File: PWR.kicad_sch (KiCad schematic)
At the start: 22 parts, among them J1 Conn_01x04_Pin, J2 Conn_01x03_Pin, J3 Conn_01x03_Pin, J4 Conn_01x03_Pin, J5 Conn_01x03_Pin, J6 Conn_01x04_Pin, U1 LM66100DCK, U2 XC6206P332MR

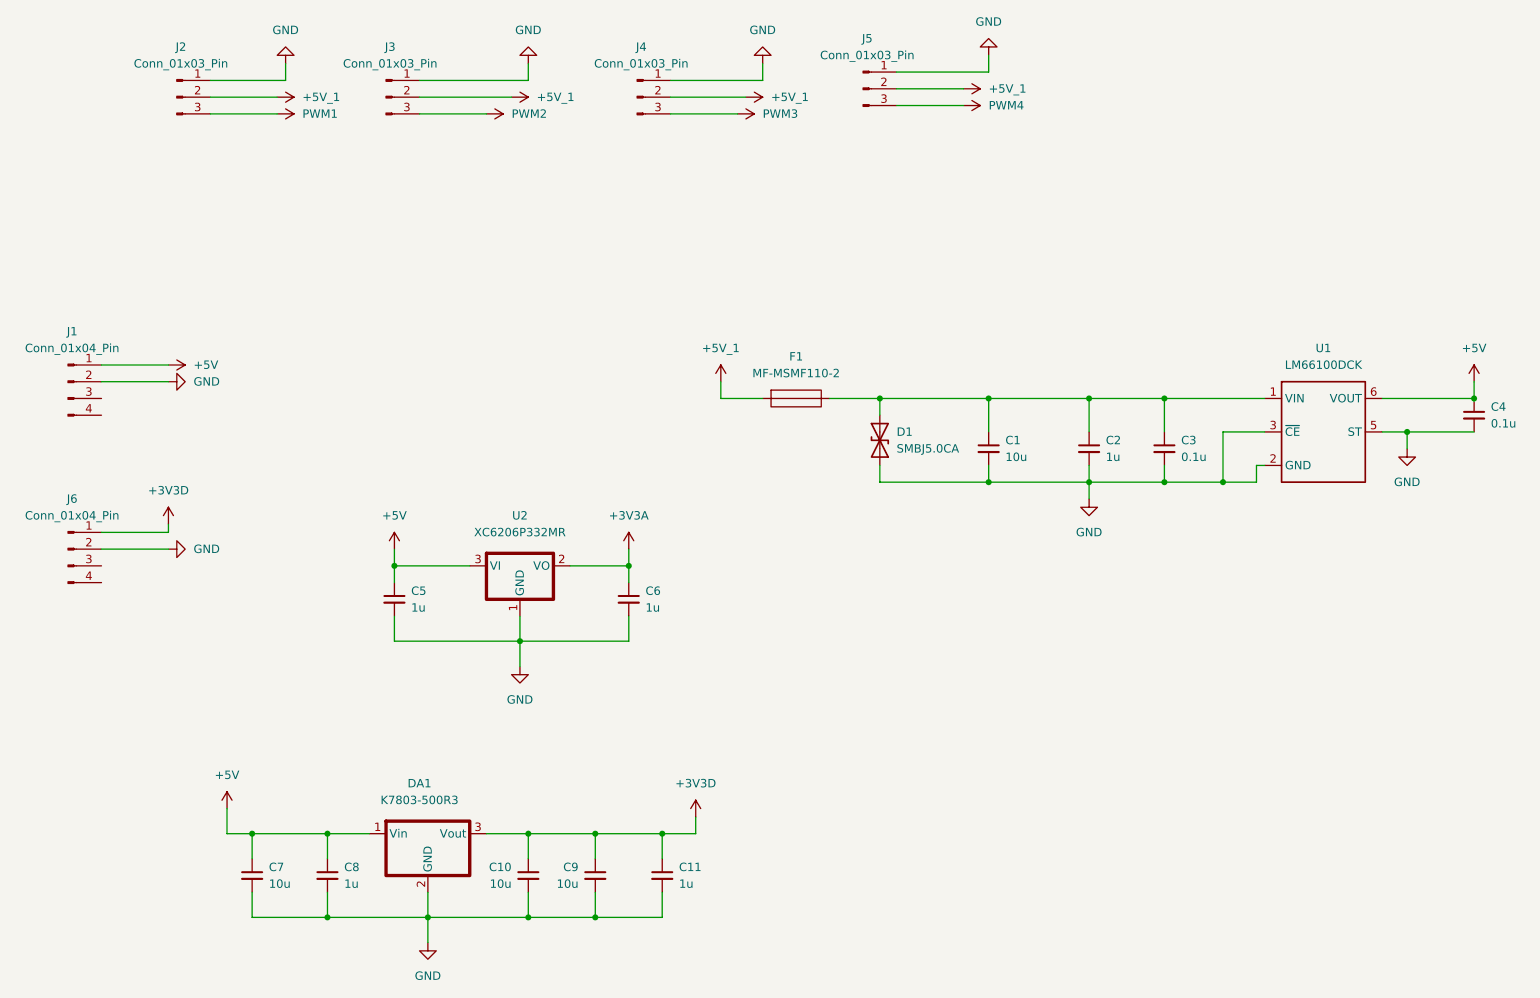
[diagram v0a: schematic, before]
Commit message: feat: firs complete version schemattic
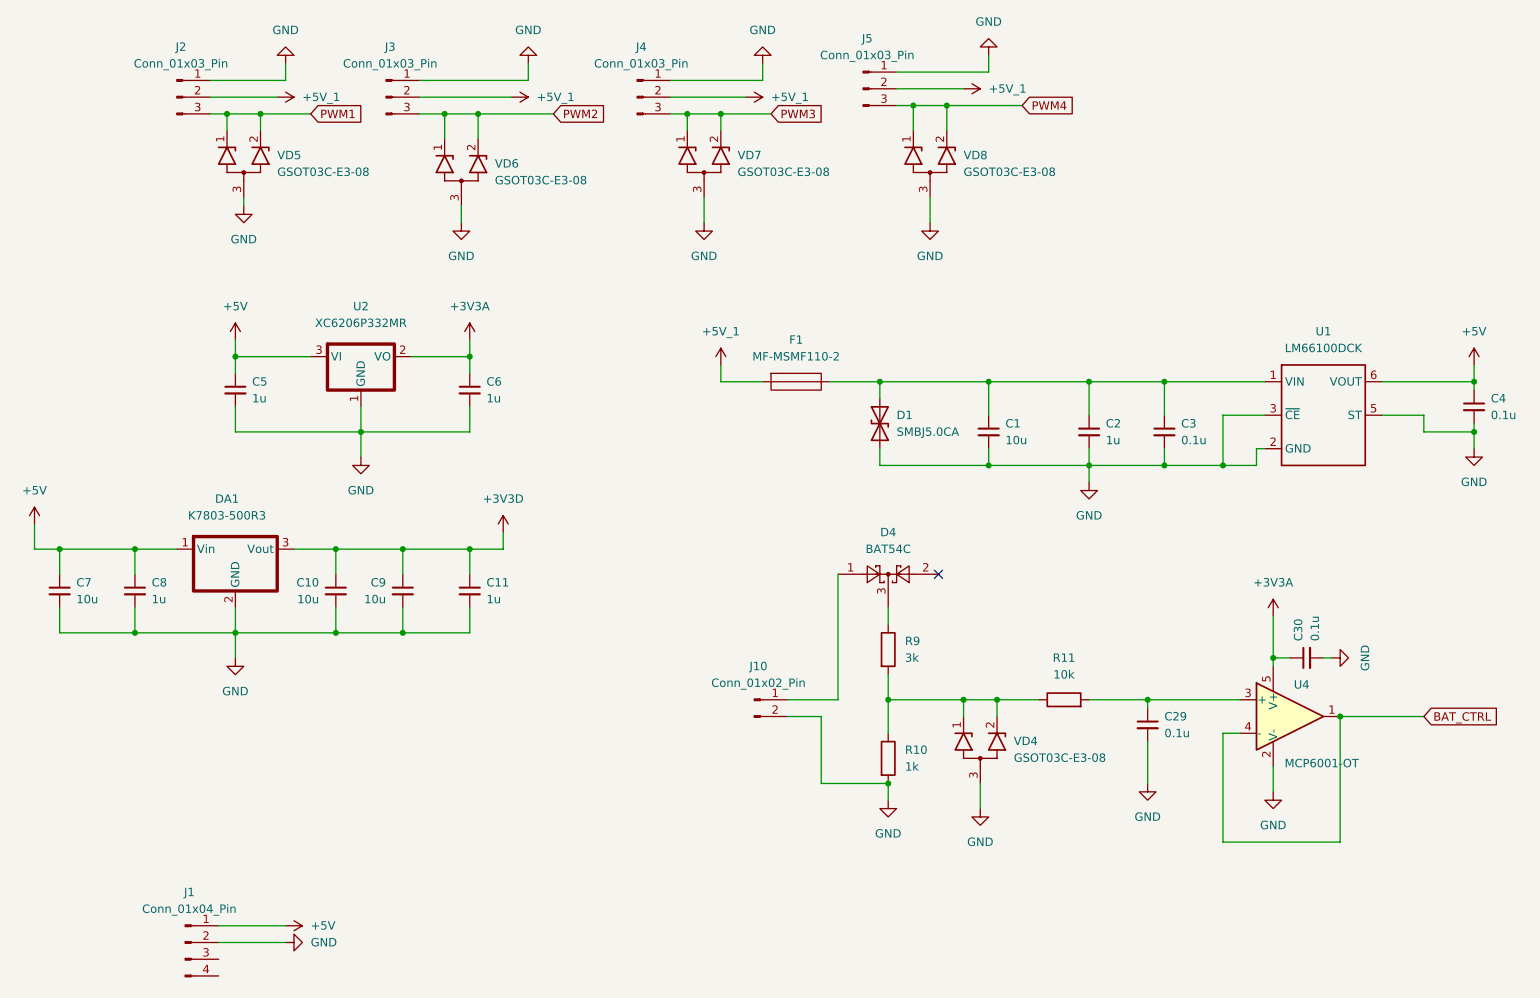
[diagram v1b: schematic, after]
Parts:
- removed J6: Conn_01x04_Pin, Connector_PinSocket_2.54mm:PinSocket_1x04_P2.54mm_Vertical, symbol Connector:Conn_01x04_Pin
- added C29, C30: 0.1u, Capacitor_SMD:C_0805_2012Metric_Pad1.18x1.45mm_HandSolder, symbol Device:C_Small
- added D4: BAT54C, Package_TO_SOT_SMD:SOT-23_Handsoldering, symbol Diode:BAT54C
- added J10: Conn_01x02_Pin, Connector_Hirose:Hirose_DF13-02P-1.25DSA_1x02_P1.25mm_Vertical, symbol Connector:Conn_01x02_Pin
- added R10: 1k, Resistor_SMD:R_0805_2012Metric_Pad1.20x1.40mm_HandSolder, symbol Device:R
- added R11: 10k, Resistor_SMD:R_0805_2012Metric_Pad1.20x1.40mm_HandSolder, symbol Device:R
- added R9: 3k, Resistor_SMD:R_0805_2012Metric_Pad1.20x1.40mm_HandSolder, symbol Device:R
- added U4: MCP6001-OT, Package_TO_SOT_SMD:SOT-23-5, symbol Amplifier_Operational:MCP6001-OT
- added VD4, VD5, VD6, VD7, VD8: GSOT03C-E3-08, Package_TO_SOT_SMD:SOT-23_Handsoldering, symbol TWS:GSOT03C-E3-08
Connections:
- net +3V3A: now also C30.1, U4.5 (V+)
- net GND: now also C29.2, C30.2, J10.2 (Pin_2), R10.2, U4.2 (V-), VD4.3 (A), VD5.3 (A), VD6.3 (A), VD7.3 (A), VD8.3 (A)
- net PWM1: now also VD5.1 (K1), VD5.2 (K2)
- net PWM2: now also VD6.1 (K1), VD6.2 (K2)
- net PWM3: now also VD7.1 (K1), VD7.2 (K2)
- net PWM4: now also VD8.1 (K1), VD8.2 (K2)
- new net: R10.1, R11.1, R9.2, VD4.1 (K1), VD4.2 (K2)
- new net: C29.1, R11.2, U4.3 (+)
- new net: D4.3, R9.1
- new net: D4.1, J10.1 (Pin_1)
- new net BAT_CTRL: U4.1, U4.4 (-)
- no-connect marks 0 -> 1
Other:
- moved on the sheet: C1, C10, C11, C2, C3, C4, C5, C6, C7, C8, C9, D1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
